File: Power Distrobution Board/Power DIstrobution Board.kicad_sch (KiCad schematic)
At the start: 2 parts, among them J2 AT15-6P-BM01GRY, J5 ATM15-12PA-BM03

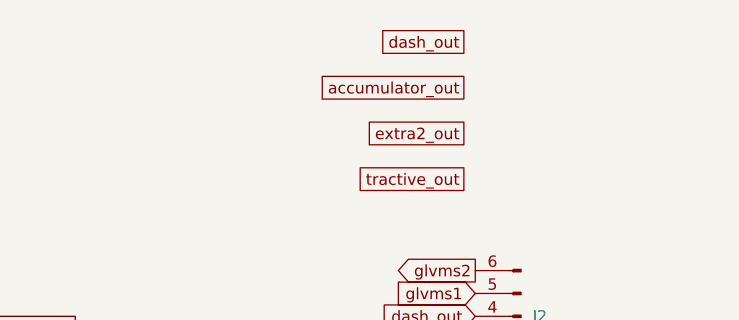
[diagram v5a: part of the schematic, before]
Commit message: changes to move to pc
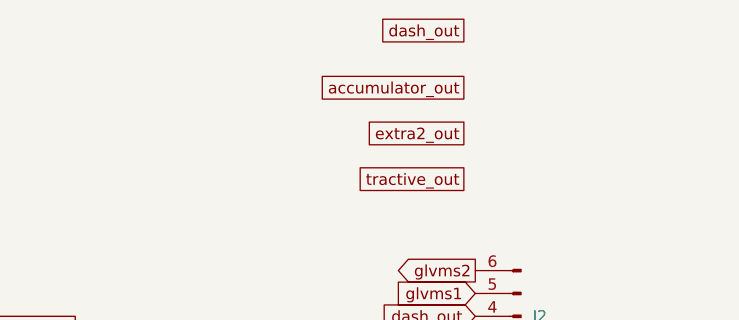
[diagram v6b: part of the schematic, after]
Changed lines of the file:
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@@
 	(global_label "dash_out"
 		(shape passive)
-		(at 266.7 38.1 180)
+		(at 266.7 36.83 180)
 		(fields_autoplaced yes)
 		(effects
@@
 		)
 		(property "Intersheetrefs" "${INTERSHEET_REFS}"
-			(at 256.3597 38.1 0)
+			(at 256.3597 36.83 0)
 			(effects
 				(font
@@
 		(length 2.54)
 		(shape round)
-		(at 266.7 38.1 270)
+		(at 266.7 36.83 270)
 		(fields_autoplaced yes)
 		(effects
@@
 			(justify right bottom)
 		)
-		(property "Netclass" "3A"
-			(at 269.24 37.4015 90)
+		(property "Netclass" "3a"
+			(at 269.24 36.1315 90)
 			(effects
 				(font
@@
 			(justify right bottom)
 		)
-		(property "Netclass" "10A"
+		(property "Netclass" "10a"
 			(at 269.24 47.5615 90)
 			(effects
@@
 			(justify right bottom)
 		)
-		(property "Netclass" "10A"
+		(property "Netclass" "10a"
 			(at 269.24 52.6415 90)
 			(effects
@@
 			(justify right bottom)
 		)
-		(property "Netclass" "3A"
+		(property "Netclass" "17a"
 			(at 269.24 42.4815 90)
 			(effects

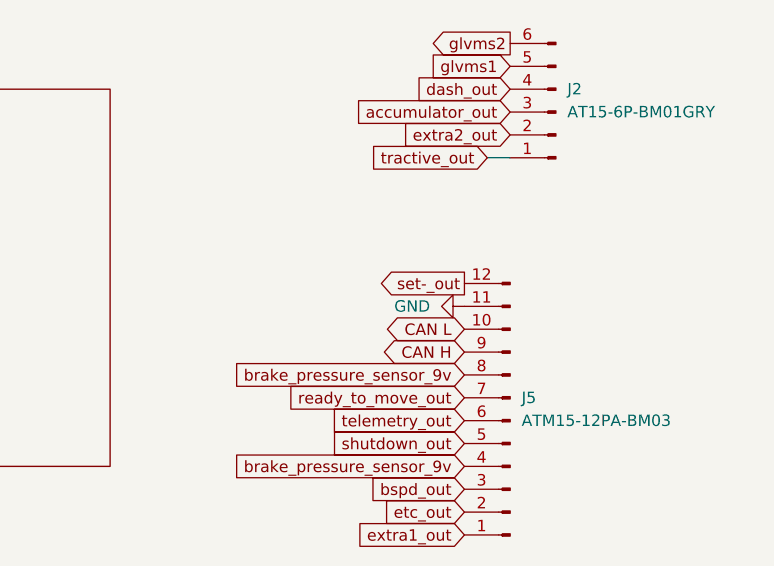
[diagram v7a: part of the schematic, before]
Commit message: v2.2
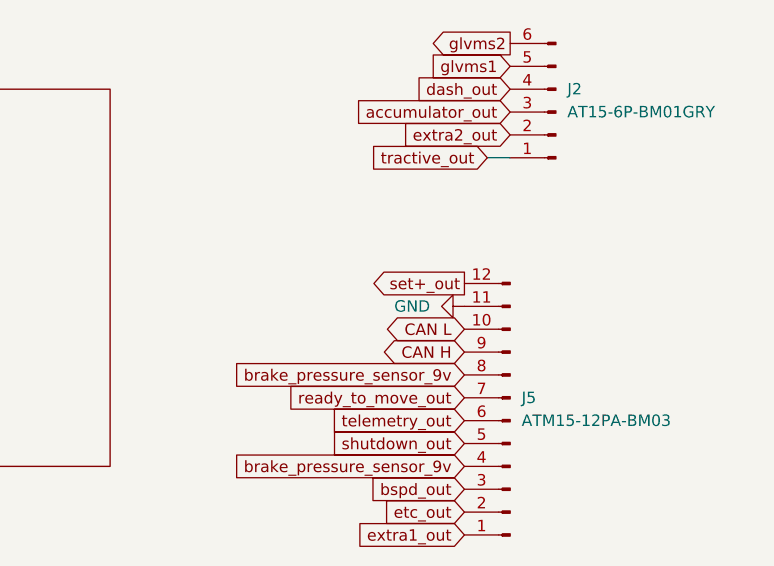
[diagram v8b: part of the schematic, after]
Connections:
- net set-_out renamed set+_out
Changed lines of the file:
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@@
 		)
 	)
-	(global_label "set-_out"
+	(global_label "set+_out"
 		(shape output)
 		(at 262.89 90.17 180)
